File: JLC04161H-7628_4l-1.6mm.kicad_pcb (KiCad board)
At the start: 2 copper layers, 24 x 24 mm, 0 parts

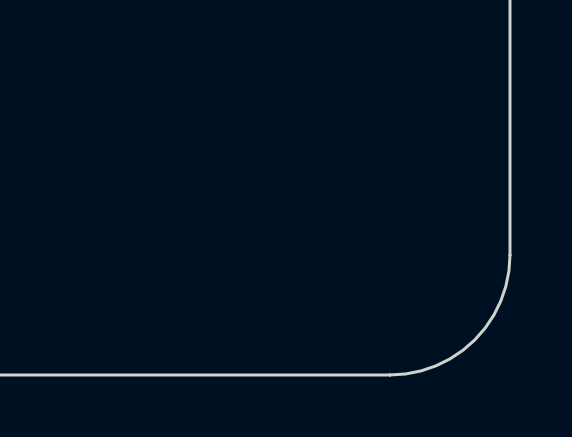
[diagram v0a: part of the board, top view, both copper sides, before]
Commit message: update stack
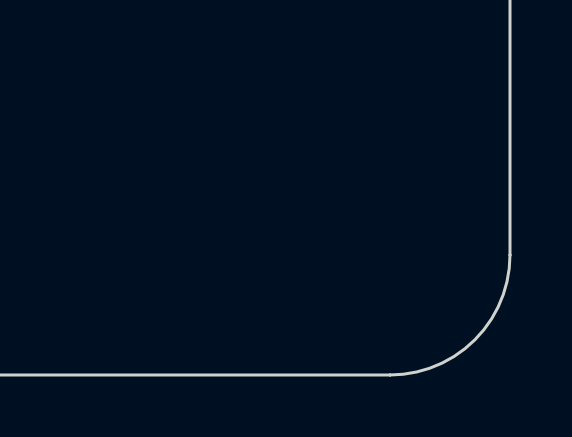
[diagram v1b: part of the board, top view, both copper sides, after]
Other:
- copper layers 2 -> 4
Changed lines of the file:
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@@
 	(generator_version "8.0")
 	(general
-		(thickness 1)
+		(thickness 1.5962)
 		(legacy_teardrops no)
 	)
@@
 		(date "SET!!!")
 		(rev "VERV")
-		(company "ELT")
+		(company "SET!!!")
 		(comment 2 "SET!!!")
 		(comment 3 "SET!!!")
@@
 	(layers
 		(0 "F.Cu" signal)
+		(1 "In1.Cu" power)
+		(2 "In2.Cu" power)
 		(31 "B.Cu" signal)
 		(32 "B.Adhes" user "B.Adhesive")
@@
 			(layer "F.Mask"
 				(type "Top Solder Mask")
-				(thickness 0.01)
+				(thickness 0.005)
 			)
 			(layer "F.Cu"
@@
 			)
 			(layer "dielectric 1"
+				(type "prepreg")
+				(thickness 0.2104 locked)
+				(material "7628")
+				(epsilon_r 4.4)
+				(loss_tangent 0.002)
+			)
+			(layer "In1.Cu"
+				(type "copper")
+				(thickness 0.0152)
+			)
+			(layer "dielectric 2"
 				(type "core")
 				(color "FR4 natural")
-				(thickness 0.91)
+				(thickness 1.065 locked)
 				(material "FR4")
-				(epsilon_r 4.5)
+				(epsilon_r 4.6)
 				(loss_tangent 0.02)
+			)
+			(layer "In2.Cu"
+				(type "copper")
+				(thickness 0.0152)
+			)
+			(layer "dielectric 3"
+				(type "prepreg")
+				(thickness 0.2104 locked)
+				(material "7628")
+				(epsilon_r 4.4)
+				(loss_tangent 0.002)
 			)
 			(layer "B.Cu"
@@
 			(layer "B.Mask"
 				(type "Bottom Solder Mask")
-				(thickness 0.01)
+				(thickness 0.005)
 			)
 			(layer "B.Paste"
@@
 		(layer "Dwgs.User")
 	)
+	(gr_arc
+		(start 34.000001 54.000001)
+		(mid 31.171573 52.828428)
+		(end 30 50)
+		(stroke
+			(width 0.1)
+			(type default)
+		)
+		(layer "Edge.Cuts")
+	)
+	(gr_arc
+		(start 50 30)
+		(mid 52.828428 31.171573)
+		(end 54.000001 34.000001)
+		(stroke
+			(width 0.1)
+			(type default)
+		)
+		(layer "Edge.Cuts")
+	)
 	(gr_line
 		(start 34 30)
@@
 	(gr_arc
 		(start 54 50)
-		(mid 52.828427 52.828427)
+		(mid 52.828427 52.828428)
 		(end 49.999999 54.000001)
+		(stroke
+			(width 0.1)
+			(type default)
+		)
+		(layer "Edge.Cuts")
+	)
+	(gr_line
+		(start 54 49.999999)
+		(end 54 34)
 		(stroke
 			(width 0.1)
@@
 		(layer "Edge.Cuts")
 	)
-	(gr_arc
-		(start 50 30)
-		(mid 52.828428 31.171573)
-		(end 54.000001 34.000001)
-		(stroke
-			(width 0.1)
-			(type default)
-		)
-		(layer "Edge.Cuts")
-	)
 	(gr_line
 		(start 29.999999 34.000001)
@@
 		(stroke
 			(width 0.1)
-			(type default)
-		)
-		(layer "Edge.Cuts")
-	)
-	(gr_arc
-		(start 34.000001 54.000001)
-		(mid 31.171573 52.828428)
-		(end 30 50)
-		(stroke
-			(width 0.1)
-			(type default)
-		)
-		(layer "Edge.Cuts")
-	)
-	(gr_line
-		(start 54 49.999999)
-		(end 54 34)
-		(stroke
-			(width 0.1)
